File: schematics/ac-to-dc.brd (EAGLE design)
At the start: 42.9 x 21.6 mm, 12 parts, among them IC1 12V

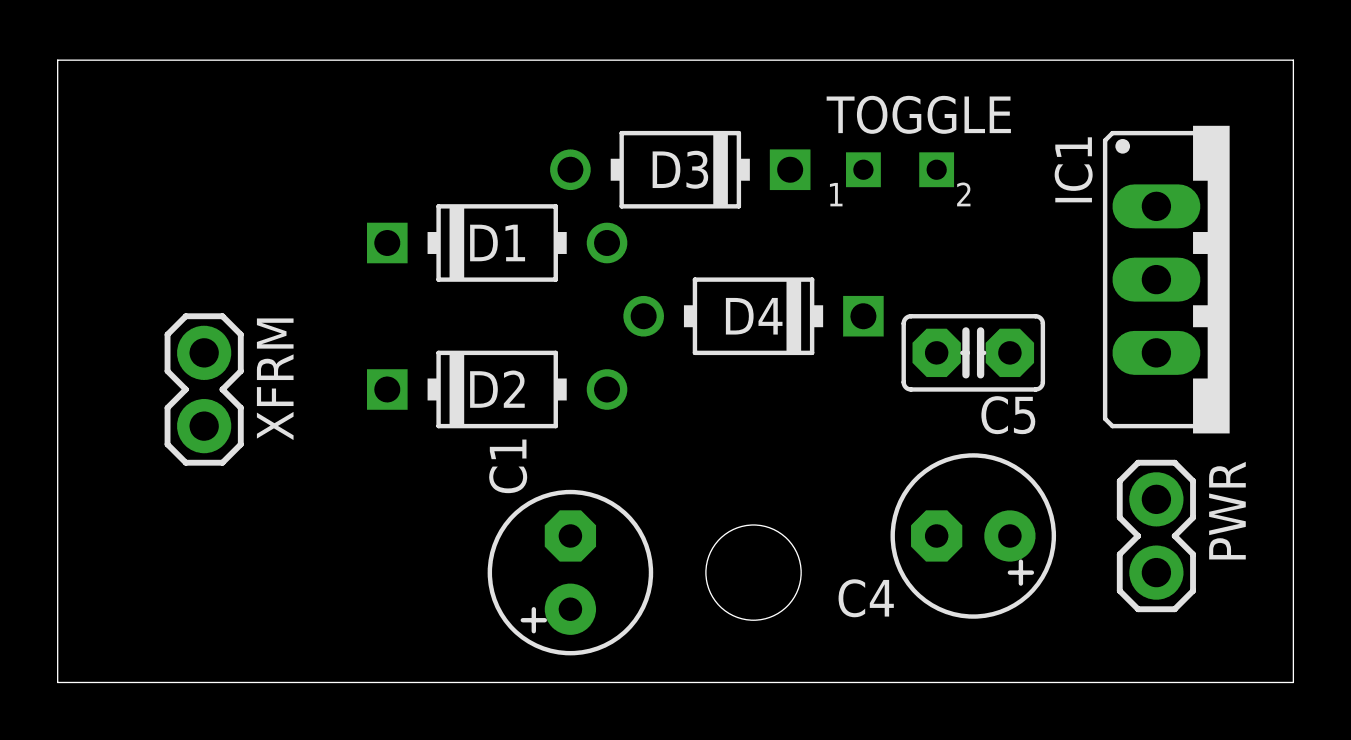
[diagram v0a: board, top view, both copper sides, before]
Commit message: Reworked the boards
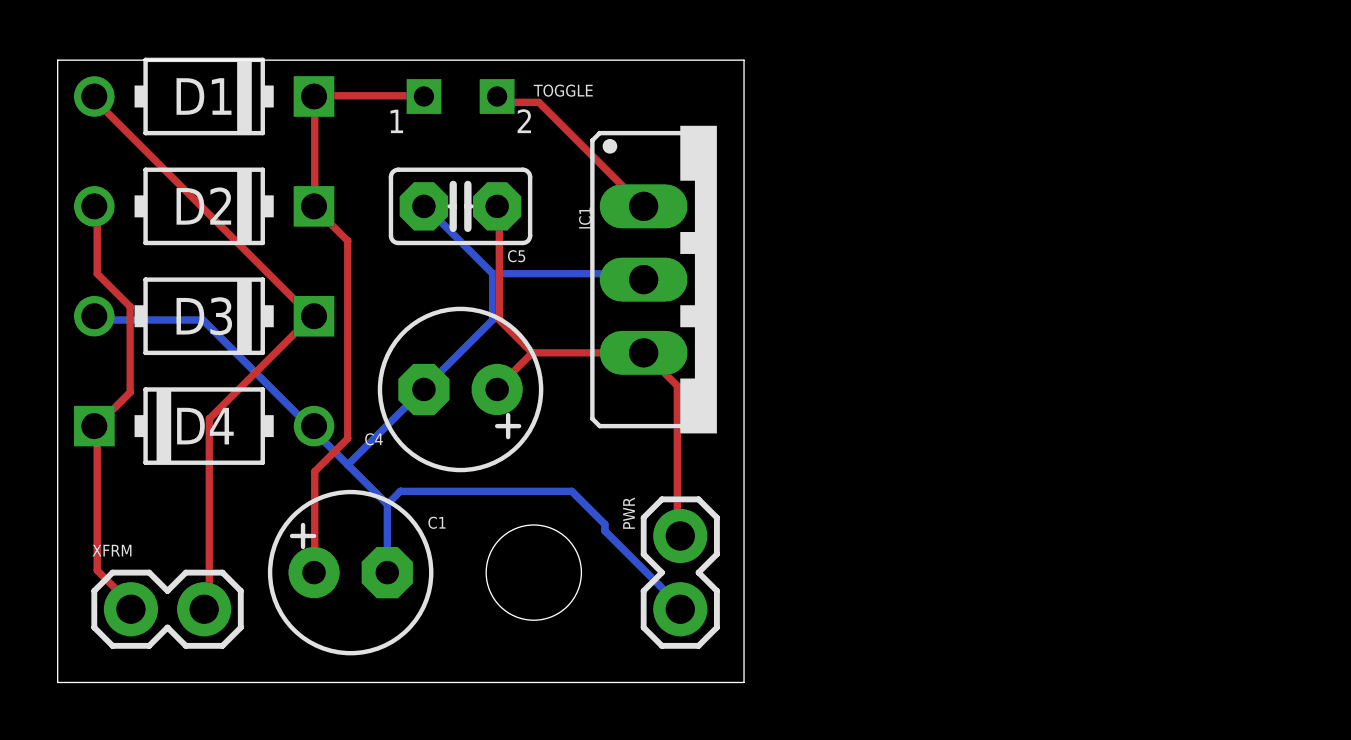
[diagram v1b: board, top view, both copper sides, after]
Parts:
- moved D4 19.4 mm to (5.08, 8.89), turned to 0 degrees
- moved C4 18.5 mm to (14.0, 10.2)
- moved C5 18.5 mm to (14.0, 16.5)
- moved IC1 17.8 mm to (22.9, 14.0)
- moved D3 17.3 mm to (5.08, 12.7)
- moved PWR 16.6 mm to (21.6, 5.08)
- moved TOGGLE 15.5 mm to (14.0, 20.3)
- moved D2 12.0 mm to (5.08, 16.5), turned to 180 degrees
- moved D1 11.4 mm to (5.08, 20.3), turned to 180 degrees
- moved XFRM 9.25 mm to (2.54, 2.54), turned to 0 degrees
- moved C1 7.62 mm to (10.2, 3.81), turned to 0 degrees
- moved JP1 7.62 mm to (16.5, 3.81)
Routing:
- net AGND: track 0.00 -> 44.9 mm
- net N$2: track 0.00 -> 22.6 mm
- net N$9: track 0.00 -> 21.3 mm
- net +12V: track 0.00 -> 18.1 mm
- net N$3: track 0.00 -> 15.6 mm
- net N$1: track 0.00 -> 6.71 mm
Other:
- board size 42.9 x 21.6 mm -> 23.8 x 21.6 mm
